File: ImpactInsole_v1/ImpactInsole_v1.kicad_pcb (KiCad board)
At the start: 2 copper layers, 44.2 x 48.3 mm, 31 parts, among them J1 503480-1800, J2 Conn_01x02, J3 USB_C_Receptacle_USB2.0_16P, U1 CD74HC4067SM96, U2 ADC081S021CIMF, U3 OPA1662D, U4 LSM6DSOXTR, U5 BQ24075RGTR, U6 ESP32-S3-WROOM-1, U7 MCP1700x-300xxTT

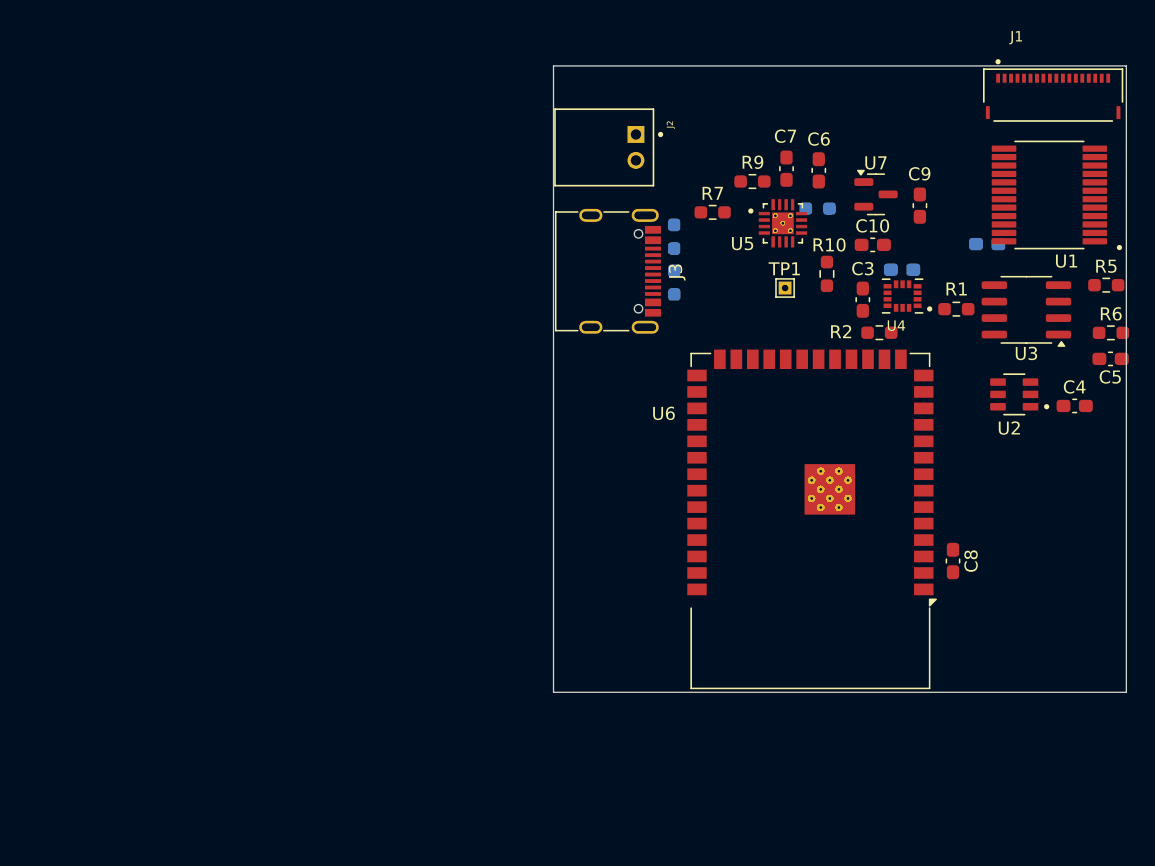
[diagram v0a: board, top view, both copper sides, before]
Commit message: idk pcb n shi
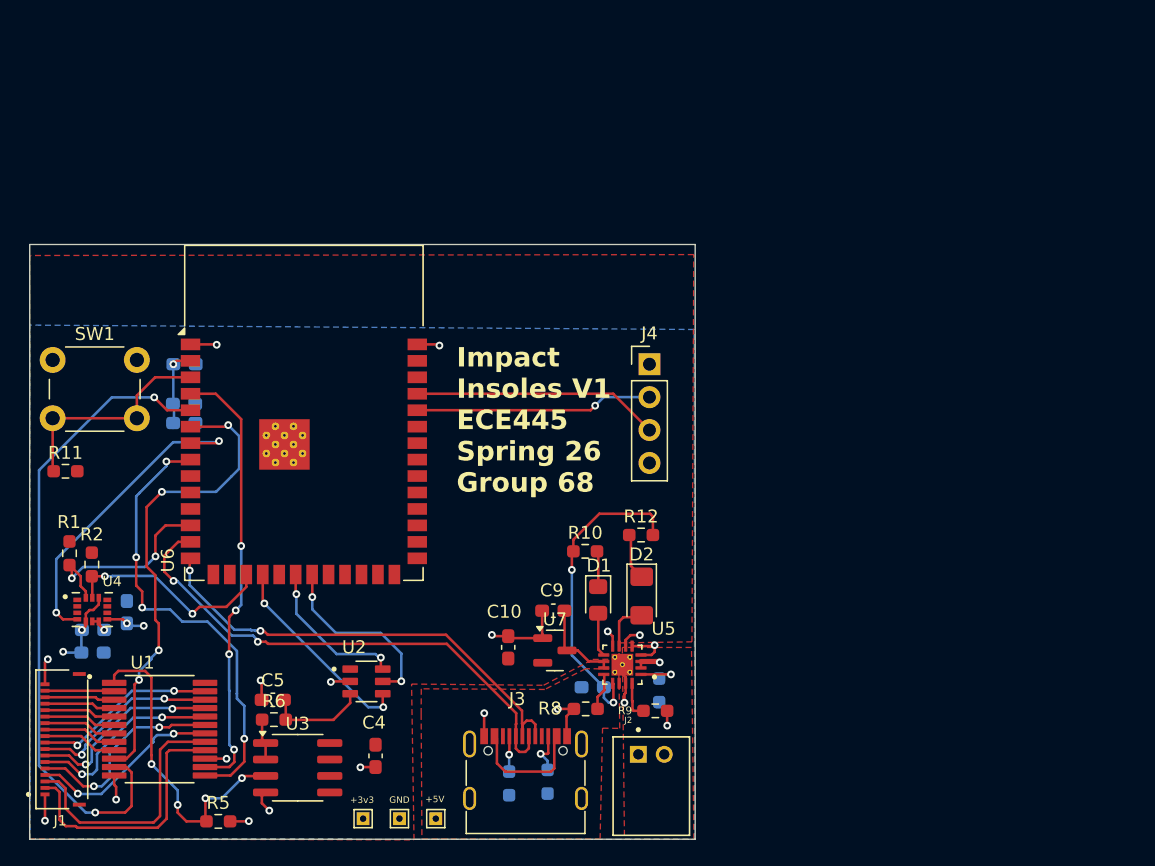
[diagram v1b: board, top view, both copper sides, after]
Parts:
- removed C1: 0.1u, Capacitor_SMD:C_0603_1608Metric_Pad1.08x0.95mm_HandSolder
- removed C2, C3: 100n, Capacitor_SMD:C_0603_1608Metric_Pad1.08x0.95mm_HandSolder
- removed C7: 10n, Capacitor_SMD:C_0603_1608Metric_Pad1.08x0.95mm_HandSolder
- removed TP1: TestPoint, TestPoint:TestPoint_THTPad_1.0x1.0mm_Drill0.5mm
- added +3v3: TestPoint, TestPoint:TestPoint_THTPad_1.0x1.0mm_Drill0.5mm, F.Cu at (102.6, 104.1)
- added +5V: TestPoint, TestPoint:TestPoint_THTPad_1.0x1.0mm_Drill0.5mm, F.Cu at (108.2, 104.1)
- added C13: 10u, Capacitor_SMD:C_0603_1608Metric_Pad1.08x0.95mm_HandSolder, B.Cu at (84.4, 88.2)
- added C14: 0.1u, Capacitor_SMD:C_0603_1608Metric_Pad1.08x0.95mm_HandSolder, B.Cu at (81.8, 91.3)
- added C15: 1u, Capacitor_SMD:C_0603_1608Metric_Pad1.08x0.95mm_HandSolder, B.Cu at (81.8, 89.5)
- added C16: 10u, Capacitor_SMD:C_0603_1608Metric_Pad1.08x0.95mm_HandSolder, B.Cu at (88.9, 69.0)
- added C17: 1u, Capacitor_SMD:C_0603_1608Metric_Pad1.08x0.95mm_HandSolder, B.Cu at (88.8, 73.6)
- added D1: LED, LED_SMD:LED_0805_2012Metric_Pad1.15x1.40mm_HandSolder, F.Cu at (120.8, 87.2)
- added D2: LED, LED_SMD:LED_1206_3216Metric_Pad1.42x1.75mm_HandSolder, F.Cu at (124.1, 86.9)
- added GND: TestPoint, TestPoint:TestPoint_THTPad_1.0x1.0mm_Drill0.5mm, F.Cu at (105.4, 104.1)
- added J4: Conn_01x04, Connector_PinHeader_2.54mm:PinHeader_1x04_P2.54mm_Vertical, F.Cu at (124.7, 69.0)
- added R11: 10k, Resistor_SMD:R_0603_1608Metric_Pad0.98x0.95mm_HandSolder, F.Cu at (79.7, 77.3)
- added R12: 3k, Resistor_SMD:R_0603_1608Metric_Pad0.98x0.95mm_HandSolder, F.Cu at (124.1, 82.2)
- added SW1: SW_Push, Button_Switch_THT:SW_PUSH_6mm_H5mm, F.Cu at (78.7, 68.7)
- C6: value 10u -> 4.7u; moved to B.Cu
- C8, R7: moved to B.Cu
- R10: value 10k -> 3k
- R8: value 2.2k -> 3k; moved to F.Cu
- R9: value 4k -> 4.4k
- moved J1 91.0 mm to (79.6, 98.0), turned to 90 degrees
- moved U1 80.1 mm to (86.9, 97.2), turned to 0 degrees
- moved R5 80.1 mm to (91.5, 104.3)
- moved R6 71.2 mm to (95.8, 96.5)
- moved R1 71.0 mm to (80.0, 83.6), turned to -90 degrees
- moved C5 69.8 mm to (95.7, 94.9)
- moved U4 67.1 mm to (81.7, 88.0), turned to 0 degrees
- moved U3 66.4 mm to (97.6, 100.2), turned to 0 degrees
- moved R2 63.4 mm to (81.7, 84.5), turned to -90 degrees
- moved C8 60.6 mm to (88.8, 72.1), turned to 0 degrees
- moved C4 60.3 mm to (103.6, 99.2), turned to -90 degrees
- moved U2 54.7 mm to (102.9, 93.5), turned to 0 degrees
- moved J2 46.9 mm to (124.9, 99.1), turned to 0 degrees
- moved R3 44.1 mm to (113.9, 101.4), turned to 90 degrees
- moved C6 43.5 mm to (120.4, 94.0), turned to 180 degrees
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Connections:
- R10 pad 2: Net-(U5-~{CHG}) -> Net-(D1-K)
- U1 pad 11: unconnected-(U1-S1-Pad11) -> /MCU/S1
- U5 pad 14: Net-(U5-TMR) -> unconnected-(U5-TMR-Pad14)
- U5 pad 5: +3V3 -> GND
- U5 pad 9: Net-(U5-~{CHG}) -> Net-(D1-A)
- U6 pad 3: +3V3 -> Net-(U6-EN)
- U6 pad 36: unconnected-(U6-RXD0-Pad36) -> /MCU/Rx_D
- U6 pad 37: unconnected-(U6-TXD0-Pad37) -> /MCU/Tx_D
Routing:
- net /MCU/S1: track 0.00 -> 50.2 mm, vias 0 -> 2
- net /MCU/USB_D_N: track 0.00 -> 40.3 mm, vias 0 -> 2
- net GND: track 0.00 -> 38.0 mm, vias 0 -> 18
- net /MCU/S2: track 0.00 -> 36.8 mm, vias 0 -> 4
- net /MCU/USB_D_P: track 0.00 -> 36.8 mm, vias 0 -> 2
- net /MCU/S3: track 0.00 -> 35.3 mm, vias 0 -> 4
- net /MCU/S0: track 0.00 -> 34.2 mm, vias 0 -> 4
- net /MCU/VDD5V: track 0.00 -> 33.7 mm, vias 0 -> 2
- net /Sensor/Mux_Out: track 0.00 -> 24.8 mm, vias 0 -> 4
- net /MCU/IMU_INT: track 0.00 -> 24.6 mm, vias 0 -> 2
- net /Sensor/sense16: track 0.00 -> 20.3 mm
- net /Sensor/sense15: track 0.00 -> 20.1 mm
- net +3V3: track 0.00 -> 19.5 mm, vias 0 -> 7
- net /MCU/Tx_D: track 0.00 -> 19.1 mm
- net /MCU/Rx_D: track 0.00 -> 18.3 mm, vias 0 -> 1
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- added copper zone on F.Cu, net +3V3
- added copper zone on F.Cu, net /MCU/VDD5V
- added copper zone on B.Cu, net GND
- added copper zone on F.Cu, net Net-(J2-Pin_1)
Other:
- board size 44.2 x 48.3 mm -> 51.4 x 45.9 mm
- board text added: "Impact Insoles V1 ECE445 Spring 26 Group 68"
